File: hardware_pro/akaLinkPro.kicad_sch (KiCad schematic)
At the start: 95 parts, among them J1 USB_C_Receptacle_USB2.0_16P, J101 ISP, J103 IDC, J3 TC2050, Q1 SI2305, Q104 AO3400A, U1 XC6206P332MR, U101 HPM5301IEG1, U102 USBLC6-2SC6, U103 SN74LVC1T45DBV, U105 TPS22918DBV, U110 SN74LVC1T45DBV, U111 SN74LVC1T45DBV, U112 SN74LVC1T45DBV, U113 SN74LVC1T45DBV, U2 LMV321, U3 SN74LVC1T45DBV, Y101 24MHz

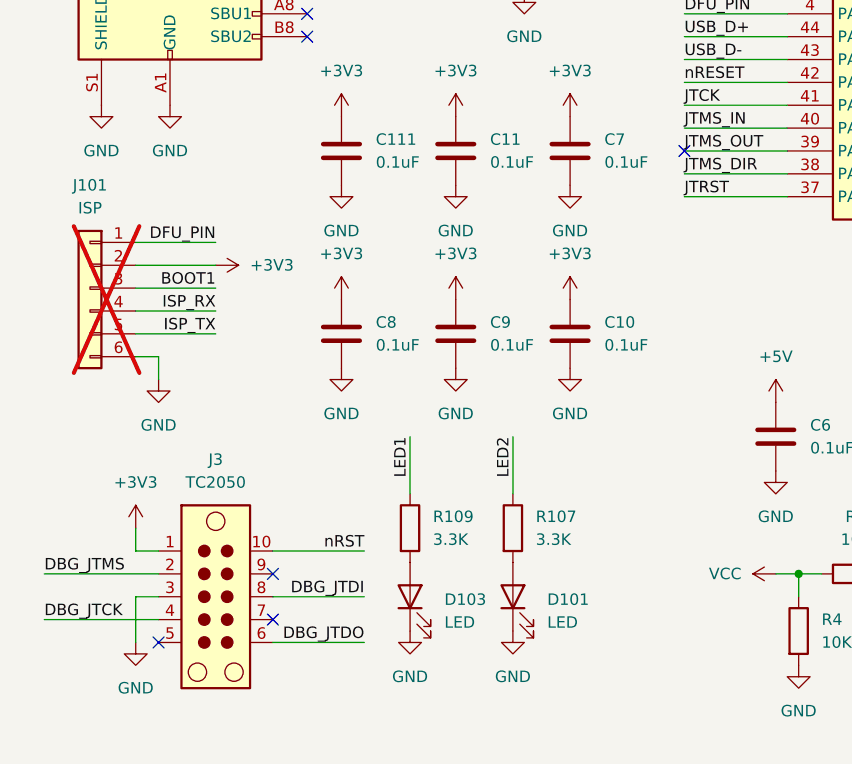
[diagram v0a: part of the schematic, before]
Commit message: update pcb
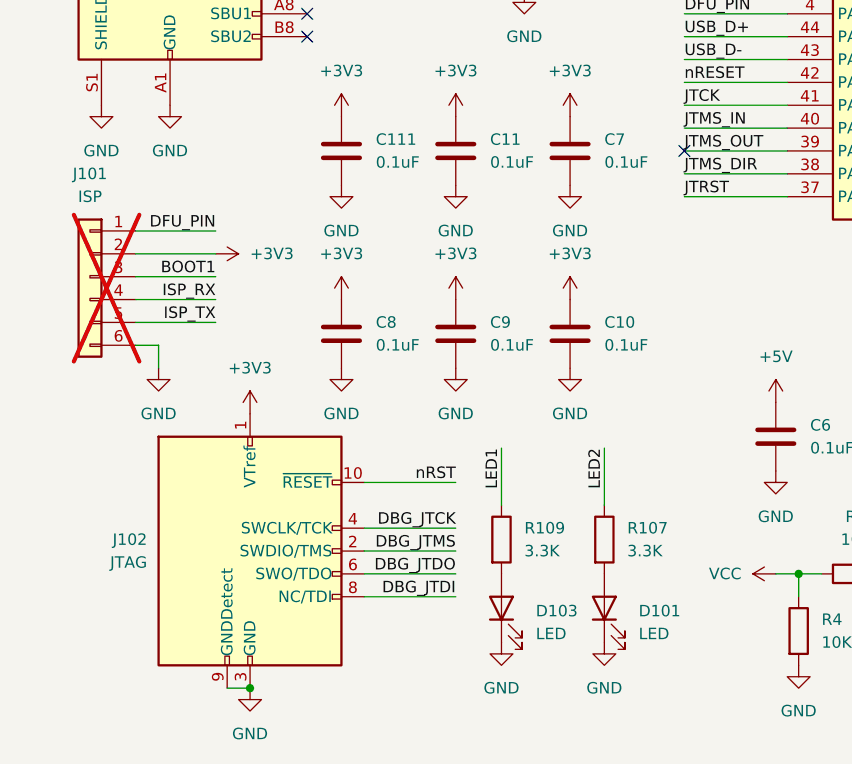
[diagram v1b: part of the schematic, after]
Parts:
- removed J3: TC2050, Connector:Tag-Connect_TC2050-IDC-NL_2x05_P1.27mm_Vertical, symbol Connector:TC2050
- added J102: JTAG, akaLink:PinHeader_2x05_P1.27mm_Vertical, symbol Connector:Conn_ARM_JTAG_SWD_10
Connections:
- net +3V3: now also J102.1 (VTref)
- net DBG_JTCK: now also J102.4 (SWCLK/TCK)
- net DBG_JTDI: now also J102.8 (NC/TDI)
- net DBG_JTDO: now also J102.6 (SWO/TDO)
- net DBG_JTMS: now also J102.2 (SWDIO/TMS)
- net GND: now also J102.3 (GND), J102.5 (GND), J102.9 (GNDDetect)
- net nRST: now also J102.10 (~{RESET})
- no-connect marks 16 -> 13
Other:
- moved on the sheet: D101, D103, J101, R107, R109
